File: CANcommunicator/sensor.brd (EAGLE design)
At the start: 33 x 26.2 mm, 31 parts, among them U1 ATSAMC21E18A-AU, U2 MCP2551

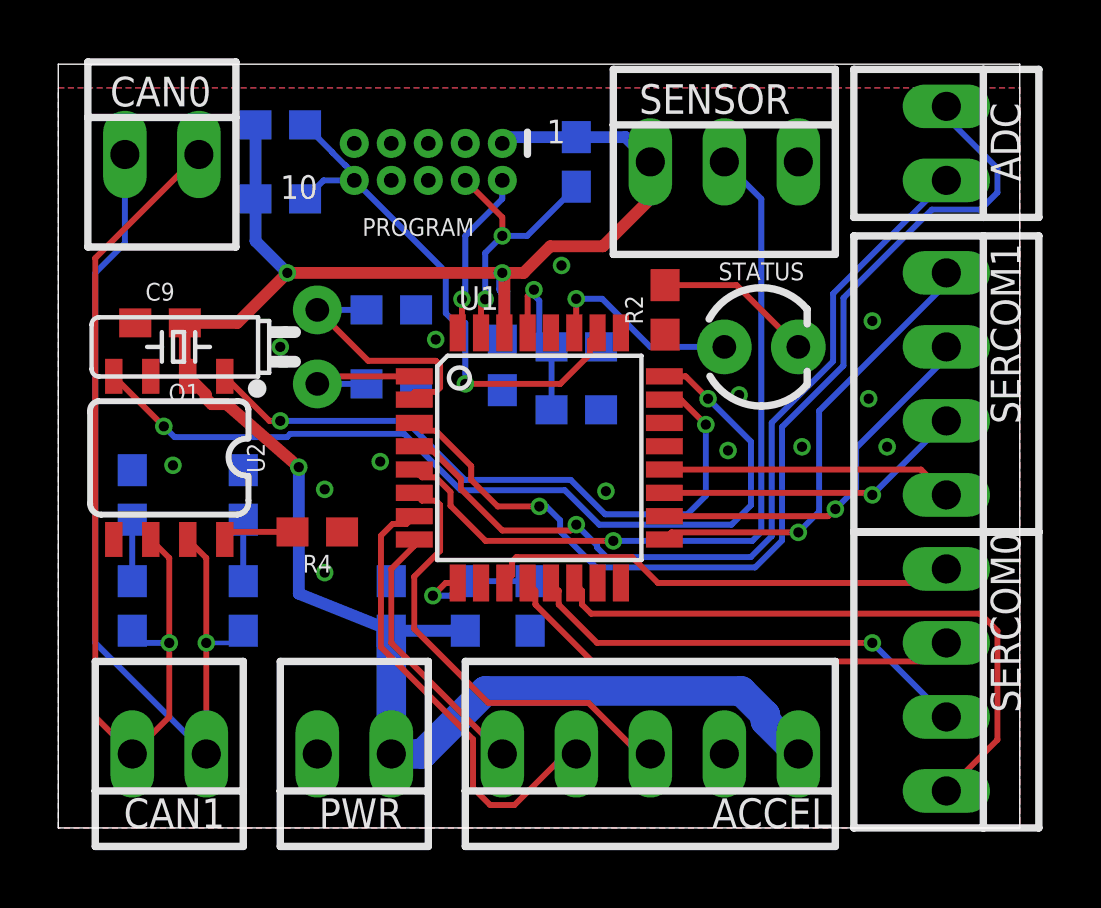
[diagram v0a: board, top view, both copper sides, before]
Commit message: moved some stuff
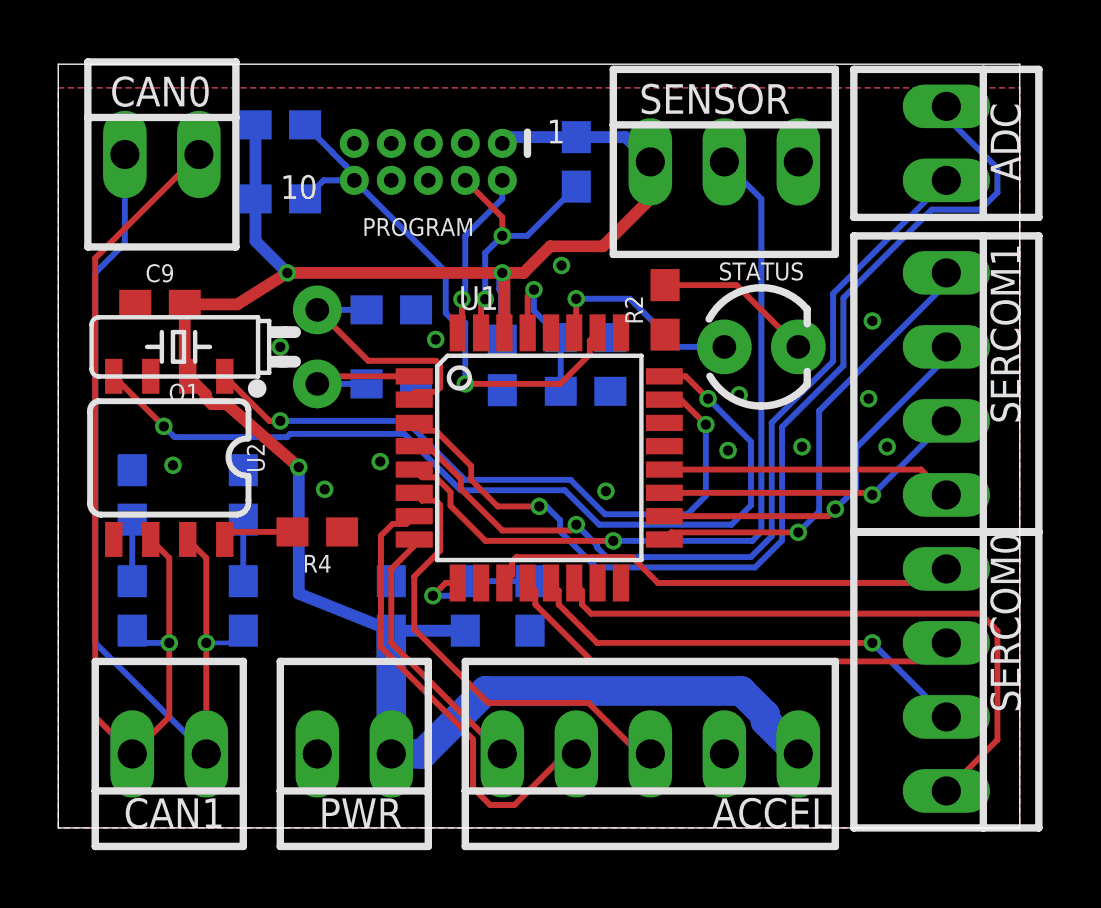
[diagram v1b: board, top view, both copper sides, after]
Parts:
- moved C5 0.71 mm to (18.1, 15.0)
- moved C9 0.64 mm to (3.49, 18.0)
- moved C4 0.45 mm to (18.1, 16.8)

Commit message: Revert changes in sensor.brd
The file in this branch is out of date and will break when we try
to merge otherwise.
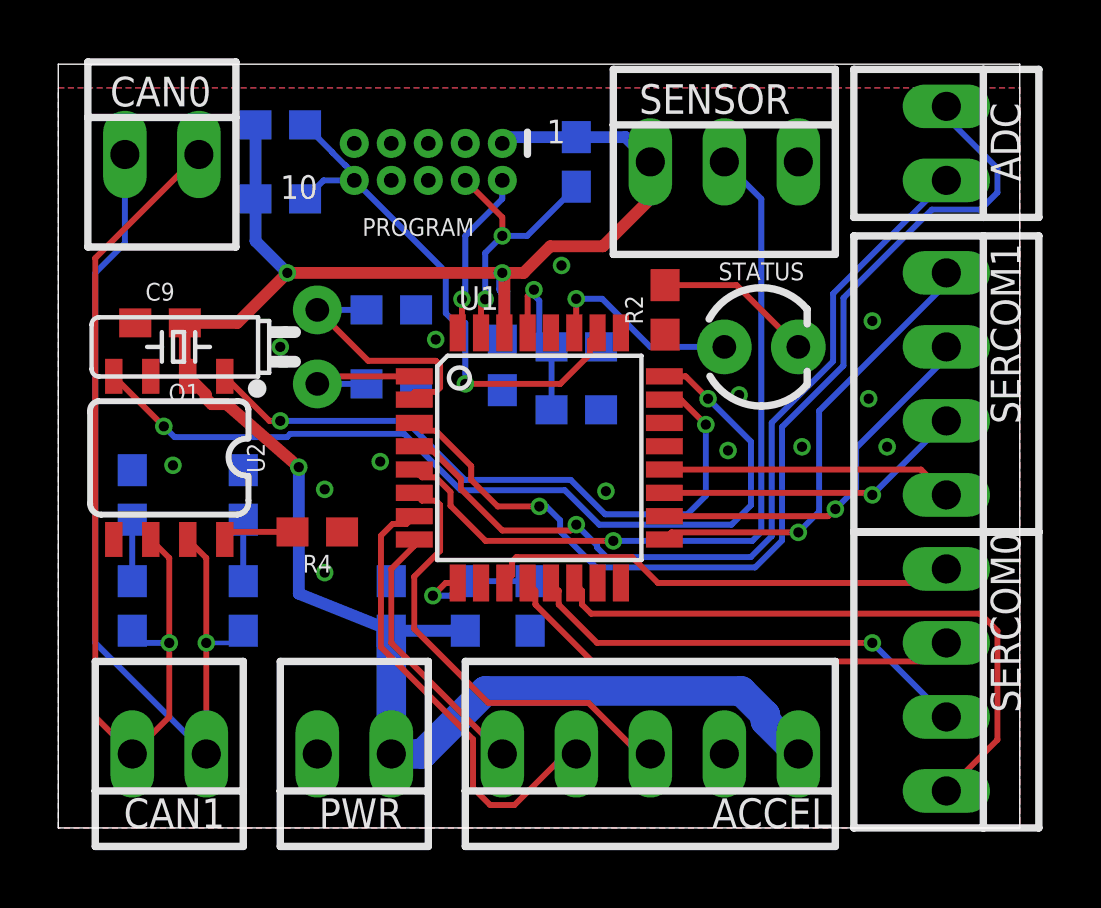
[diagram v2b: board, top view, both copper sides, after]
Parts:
- moved C5 0.71 mm to (17.8, 14.4)
- moved C9 0.64 mm to (3.49, 17.3)
- moved C4 0.45 mm to (17.8, 16.5)
